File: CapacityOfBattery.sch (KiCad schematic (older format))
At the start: 27 parts, among them J1 BATTERY, J2 DUT, Q1 IRLML6401TRPBF, Q2 IRLML6401TRPBF, Q3 IRLML6401TRPBF, Q4 IRLML6401TRPBF, Q5 IRLML6401TRPBF, Q6 SI2302, U1 NodeMCU1.0(ESP-12E)

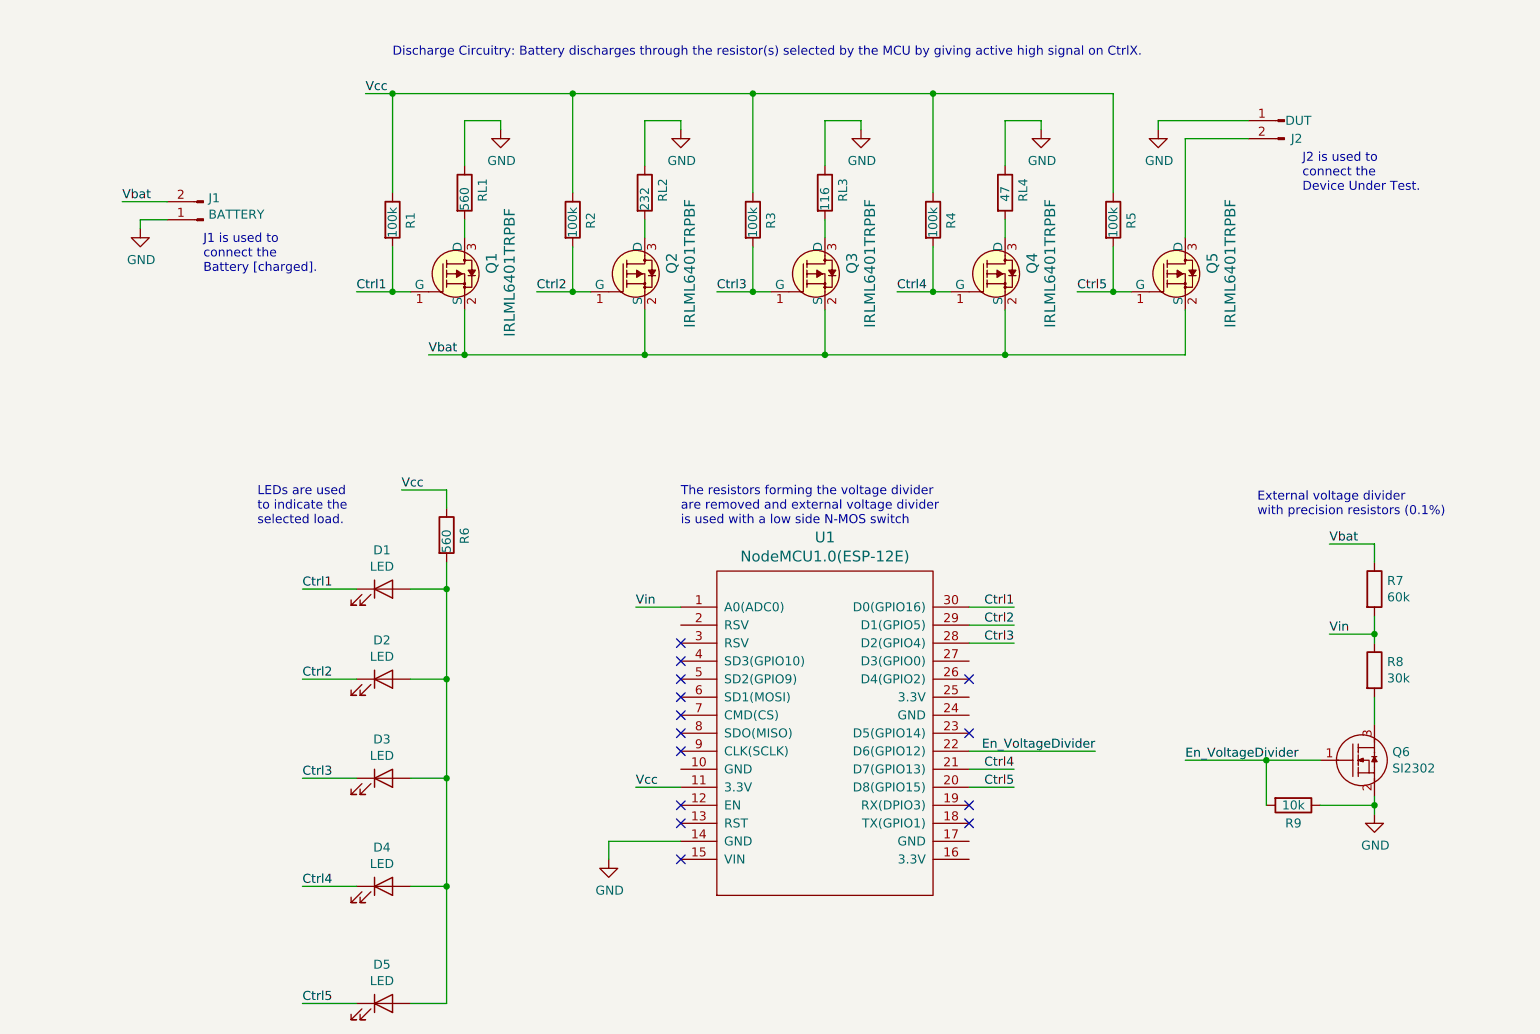
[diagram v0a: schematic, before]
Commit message: modified pcb
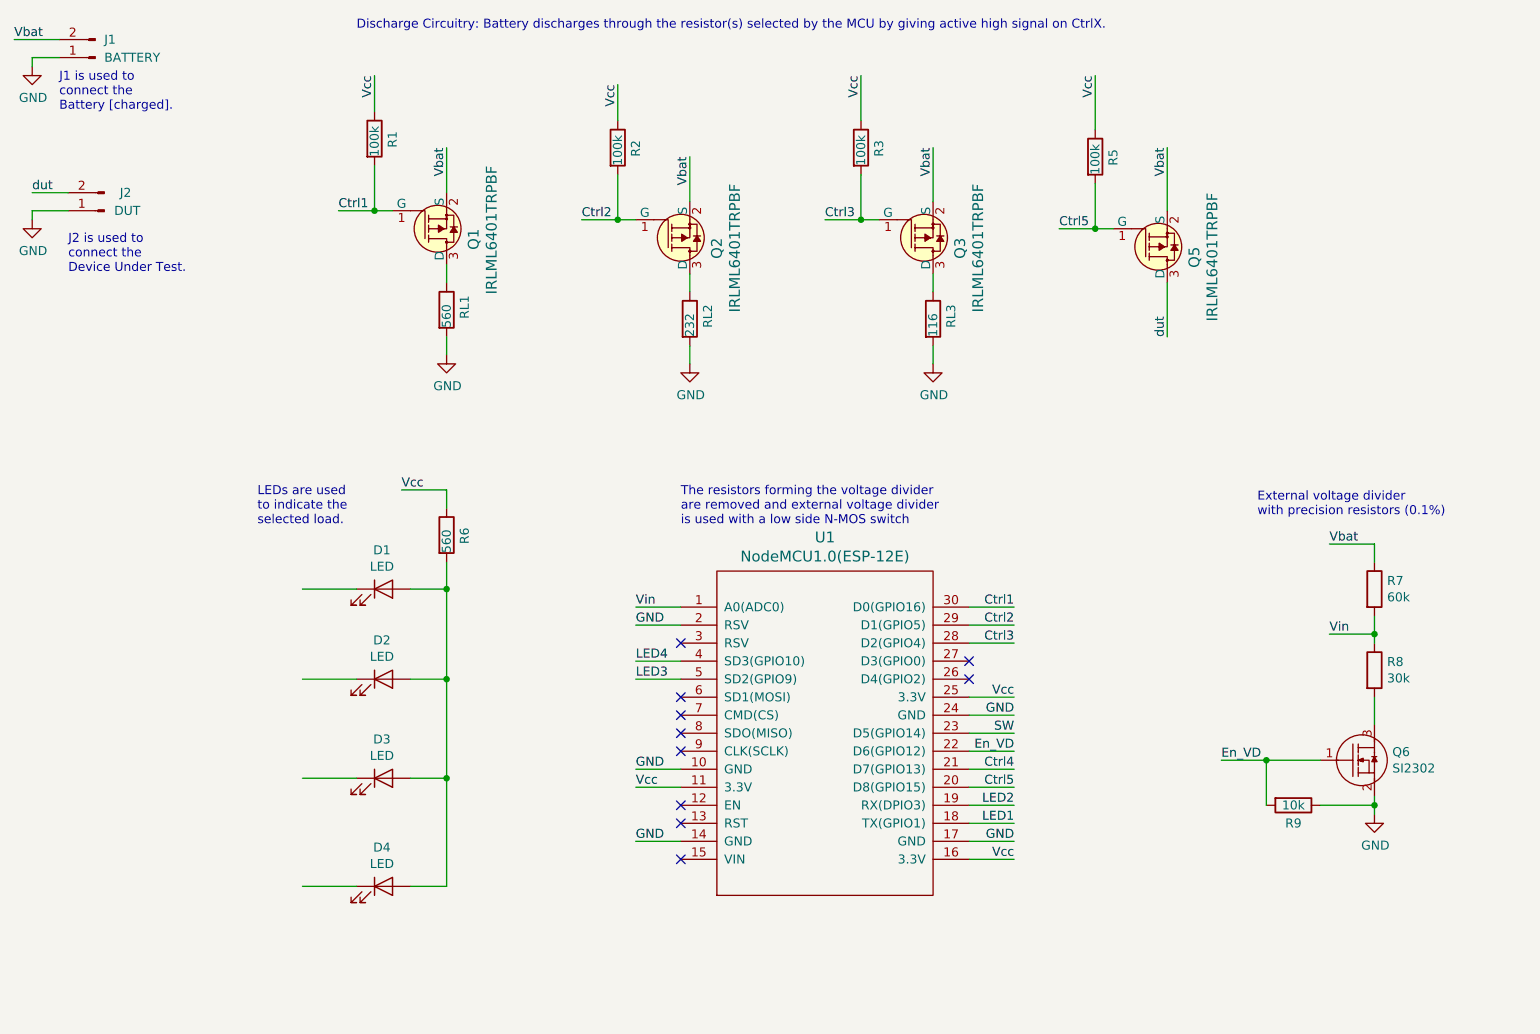
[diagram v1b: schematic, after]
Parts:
- removed D5: LED, LED_SMD:LED_0805_2012Metric_Pad1.15x1.40mm_HandSolder, symbol Device:LED
- removed Q4: IRLML6401TRPBF, Package_TO_SOT_SMD:SOT-23, symbol dk_Transistors-FETs-MOSFETs-Single:IRLML6401TRPBF
- removed R4: 100k, Resistor_SMD:R_0805_2012Metric_Pad1.15x1.40mm_HandSolder, symbol Device:R
- removed RL4: 47, Resistor_SMD:R_0805_2012Metric_Pad1.15x1.40mm_HandSolder, symbol Device:R
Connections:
- net labels added: En_VD, LED1, LED2, LED3, LED4, SW, dut
- net labels removed: En_VoltageDivider
- wire segments 97 -> 79
- no-connect marks 14 -> 10
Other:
- moved on the sheet: J1, J2, Q1, Q2, Q3, Q5, R1, R2, R3, R5, RL1, RL2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
